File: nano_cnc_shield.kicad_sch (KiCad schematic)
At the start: 18 parts, among them J1 POWER_12V, J2 LASER, J3 STEPPER_X, J4 STEPPER_Y, Q1 IRFZ44N, U1 L7805

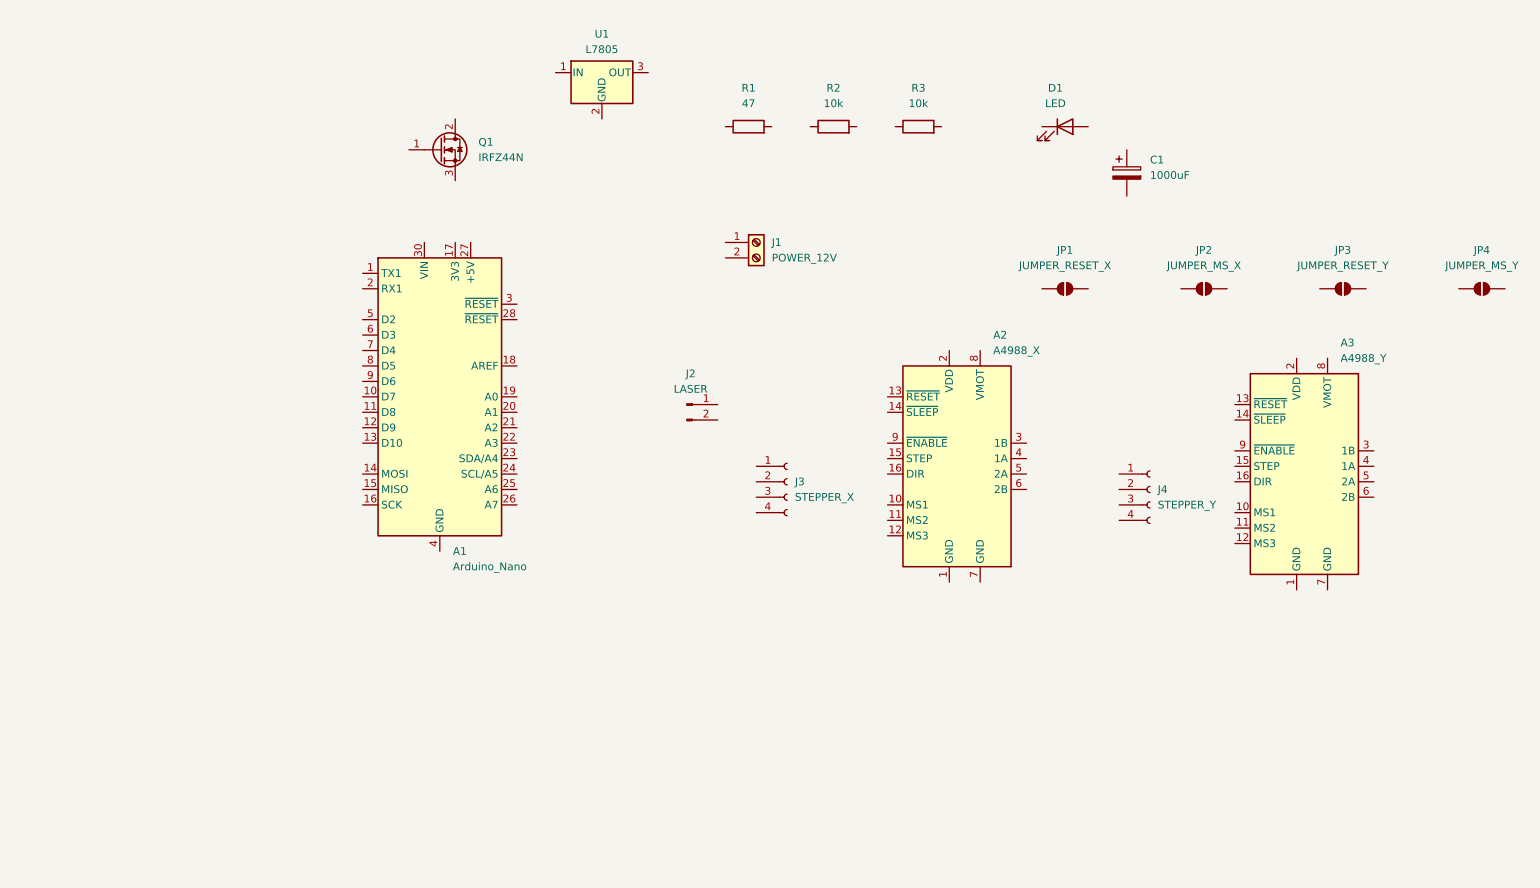
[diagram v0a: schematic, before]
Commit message: finished schematic
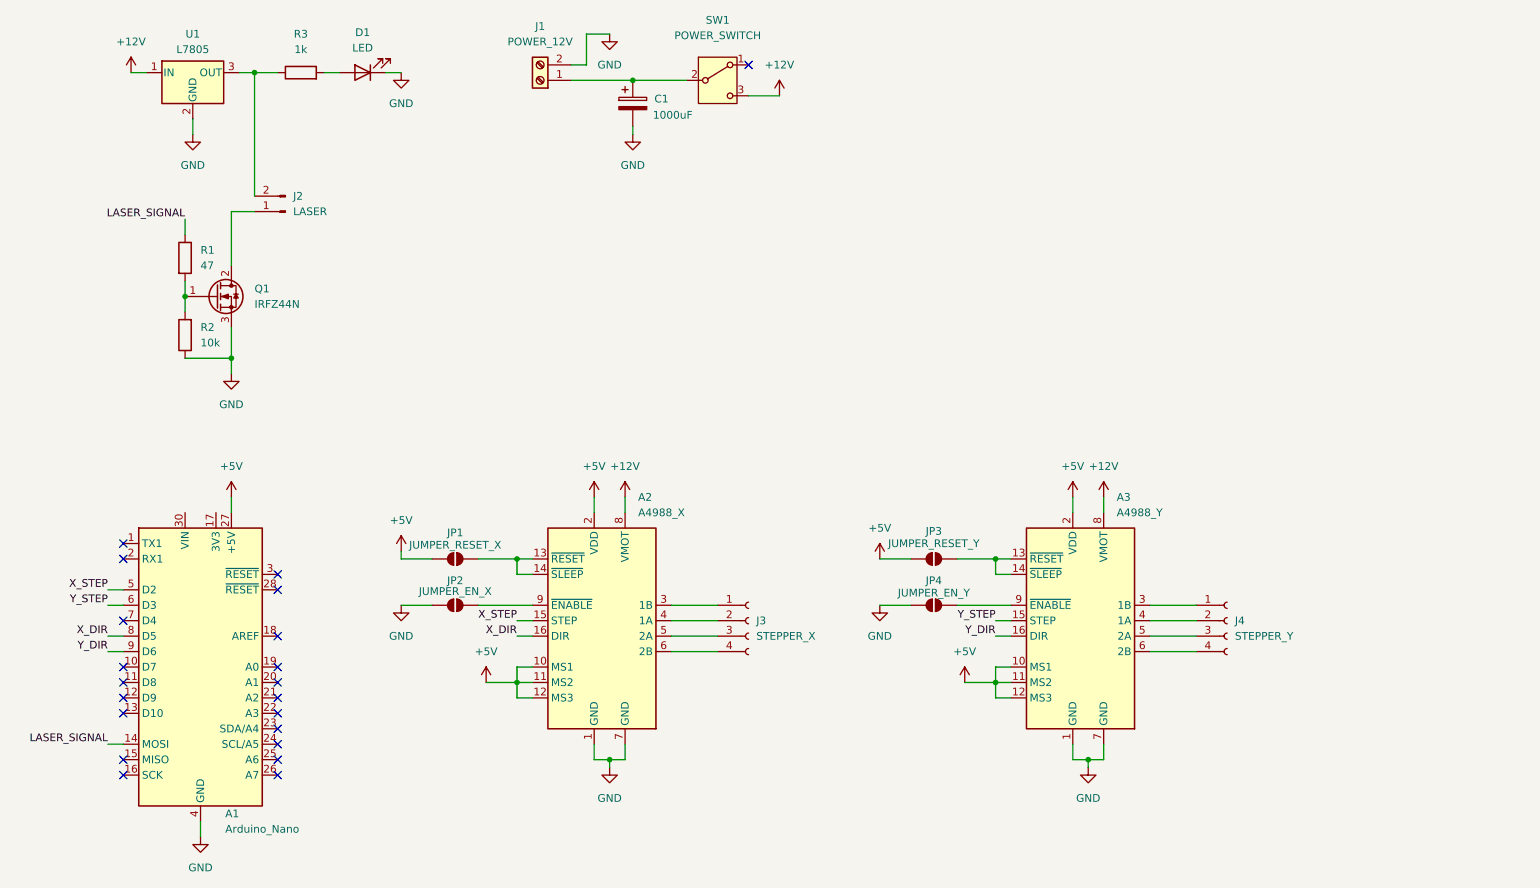
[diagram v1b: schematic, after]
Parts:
- added SW1: POWER_SWITCH, switch:SW_Slide-03_SS22T35_8.4x3.8x6.8_P2.54mm, symbol Switch:SW_SPDT
- JP2: value JUMPER_MS_X -> JUMPER_EN_X
- JP4: value JUMPER_MS_Y -> JUMPER_EN_Y
- R3: value 10k -> 1k
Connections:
- net LASER_SIGNAL: now reaches A1.14 (MOSI)
- net LASER_SIGNAL: now also R1.1
- net +5V: now reaches A1.27 (+5V)
- net +5V: now also A2.10 (MS1), A2.11 (MS2), A2.12 (MS3), A2.2 (VDD), A3.10 (MS1), A3.11 (MS2), A3.12 (MS3), A3.2 (VDD), JP1.1 (A), JP3.1 (A)
- net GND: now reaches A1.29 (GND), A1.4 (GND)
- net GND: now also A2.1 (GND), A2.7 (GND), A3.1 (GND), A3.7 (GND), C1.2, D1.1 (K), J1.2 (GND), JP2.1 (A), JP4.1 (A), Q1.3 (S), R2.1, U1.2 (GND)
- net X_STEP: now reaches A1.5 (D2)
- net X_STEP: now also A2.15 (STEP)
- net Y_STEP: now reaches A1.6 (D3)
- net Y_STEP: now also A3.15 (STEP)
- net X_DIR: now reaches A1.8 (D5)
- net X_DIR: now also A2.16 (DIR)
- net Y_DIR: now reaches A1.9 (D6)
- net Y_DIR: now also A3.16 (DIR)
- net at R2.2: now also Q1.1 (G), R1.2
- net at C1.1: now also J1.1 (V+), SW1.2 (B)
- net at JP3.2 (B): now also A3.13 (~{RESET}), A3.14 (~{SLEEP})
- net at J3.1 (Pin_1): now also A2.3 (1B)
- net at J3.2 (Pin_2): now also A2.4 (1A)
- net at J3.3 (Pin_3): now also A2.5 (2A)
- net at J3.4 (Pin_4): now also A2.6 (2B)
- net at A2.13 (~{RESET}): now also A2.14 (~{SLEEP}), JP1.2 (B)
- net +12V: now reaches A2.8 (VMOT)
- net +12V: now also A3.8 (VMOT), U1.1 (IN), SW1.3 (C)
- net at A2.9 (~{ENABLE}): now also JP2.2 (B)
- net at R3.1: now also J2.2 (Pin_2), U1.3 (OUT)
- net at R3.2: now also D1.2 (A)
- net at A3.3 (1B): now also J4.1 (Pin_1)
- net at A3.4 (1A): now also J4.2 (Pin_2)
- net at A3.5 (2A): now also J4.3 (Pin_3)
- net at A3.6 (2B): now also J4.4 (Pin_4)
- net at A3.9 (~{ENABLE}): now also JP4.2 (B)
- net at J2.1 (Pin_1): now also Q1.2 (D)
- no-connect marks 0 -> 21
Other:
- moved on the sheet: A1, A2, A3, C1, D1, J1, J2, J3, J4, JP1, JP2, JP3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
